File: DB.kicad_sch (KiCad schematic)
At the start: 6 parts

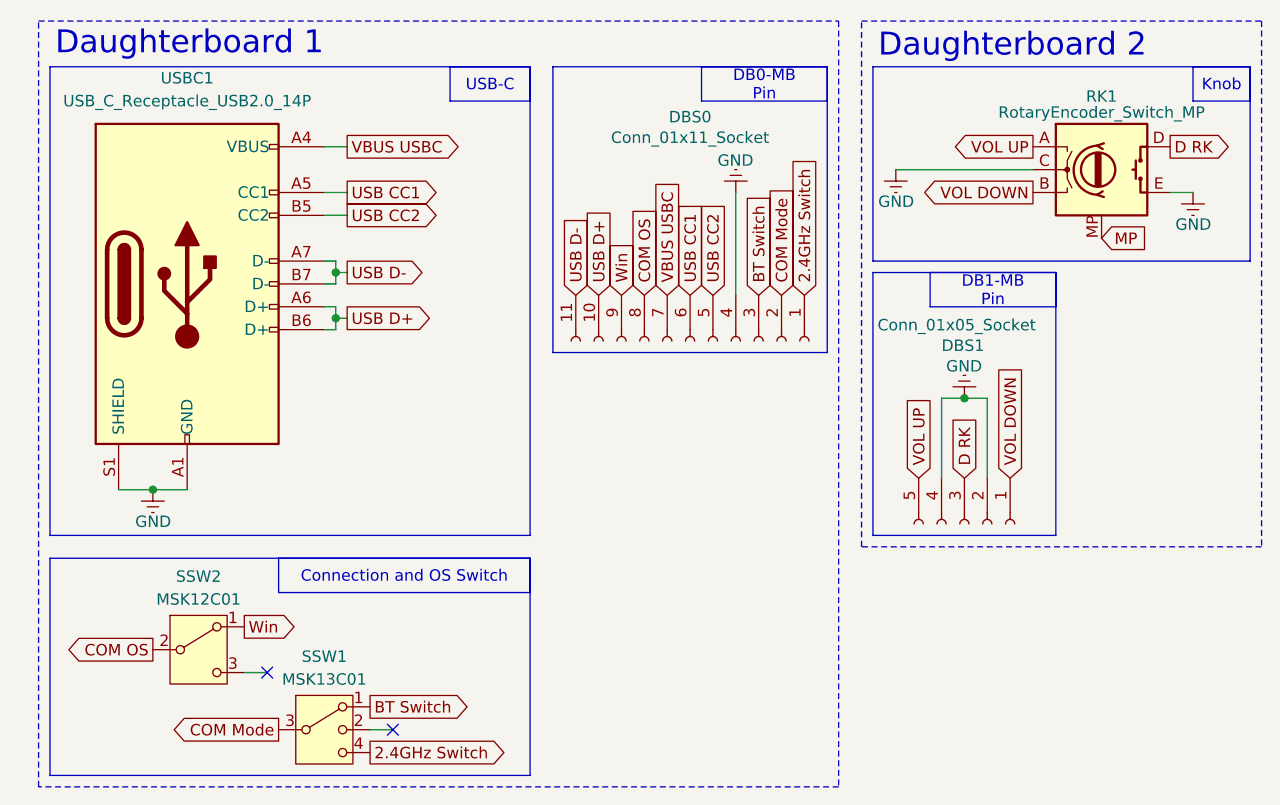
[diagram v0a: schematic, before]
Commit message: 9th commit
some minor tweak + adding production files
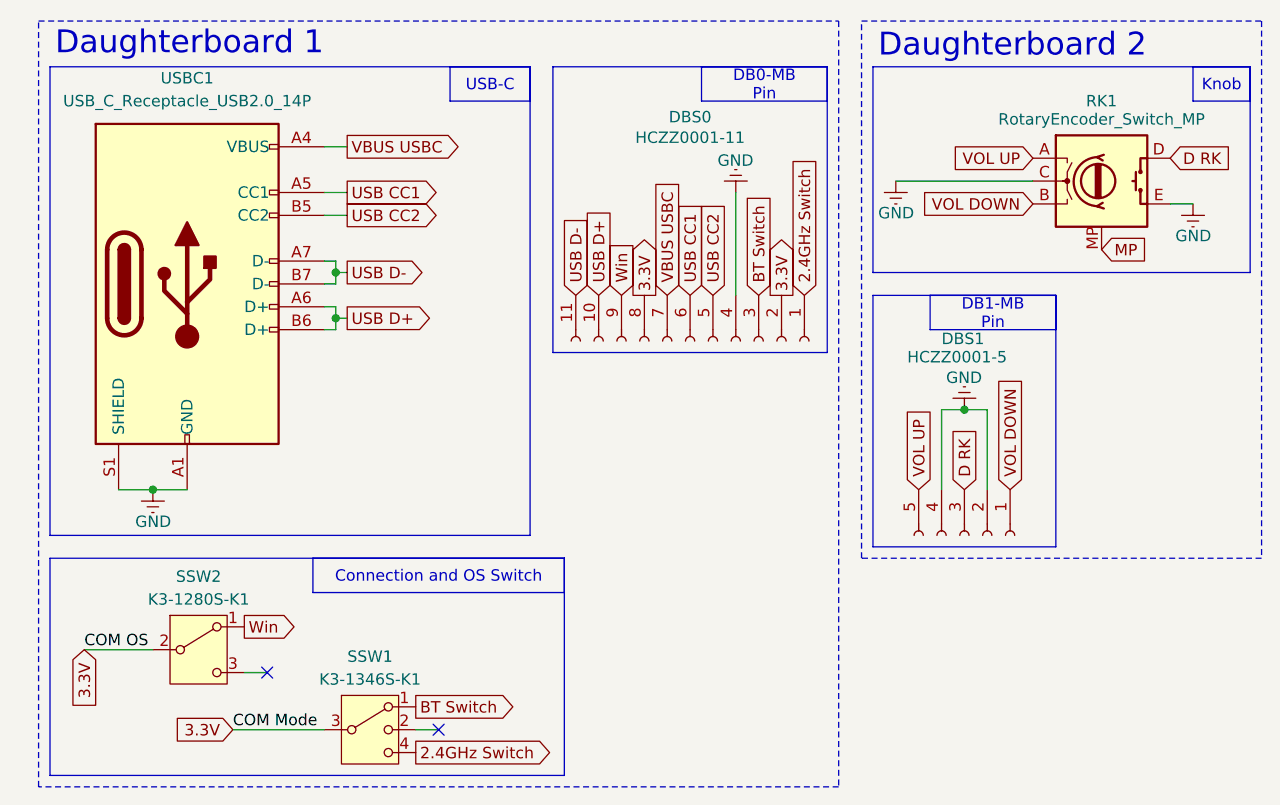
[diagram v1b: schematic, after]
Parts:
- DBS0: value Conn_01x11_Socket -> HCZZ0001-11; footprint Connector_Molex:Molex_PicoBlade_53261-1171_1x11-1MP_P1.25mm_Horizontal -> HE_Keyswitch:Hong_Cheng_HCZZ0001-11; LCSC Part (none) -> C7433462
- DBS1: value Conn_01x05_Socket -> HCZZ0001-5; footprint Connector_Molex:Molex_PicoBlade_53261-0571_1x05-1MP_P1.25mm_Horizontal -> HE_Keyswitch:Hong_Cheng_HCZZ0001-5; LCSC Part (none) -> C7433456
- RK1: footprint HE_Keyswitch:RotaryEncoder_Bourns_Vertical_PEC11J-9220F-S0015 -> HE_Keyswitch:RotaryEncoder_CTR_ED11601M-FB15A7.0-C15-202; LCSC Part (none) -> C470592
- SSW1: value MSK13C01 -> K3-1346S-K1; footprint Button_Switch_SMD:SW_SP3T_PCM13 -> HE_Keyswitch:SW_SP3T_Korean_Hroparts_Elec_K3-1346S-K1; LCSC Part (none) -> C128957
- SSW2: value MSK12C01 -> K3-1280S-K1; footprint Button_Switch_SMD:SW_SPDT_PCM12 -> HE_Keyswitch:SW_SPDT_Korean_Hroparts_Elec_K3-1280S-K1; LCSC Part (none) -> C128953
- USBC1: LCSC Part (none) -> C165948
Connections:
- net COM OS is gone; now on net 3.3V: DBS0.8 (Pin_8), SSW2.2 (B)
- net COM Mode renamed 3.3V
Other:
- moved on the sheet: DBS1, RK1, SSW1
